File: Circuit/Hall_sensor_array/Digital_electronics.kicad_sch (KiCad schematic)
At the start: 17 parts, among them J1 Conn_01x04_Female, U277 4040

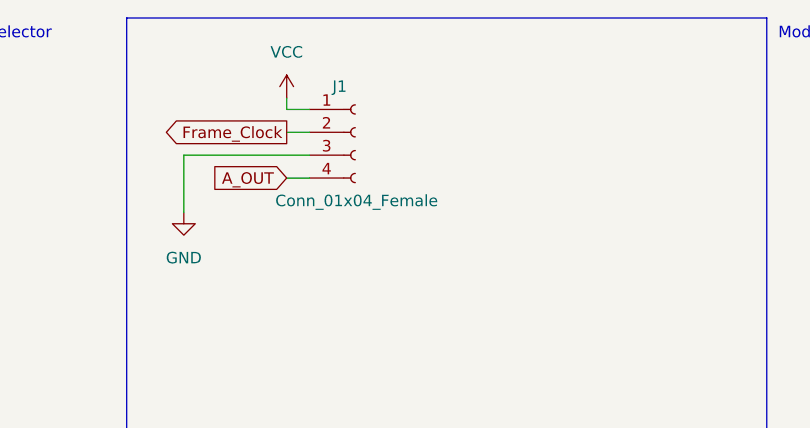
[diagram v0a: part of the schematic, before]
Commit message: Major update! New pcb
i did some work
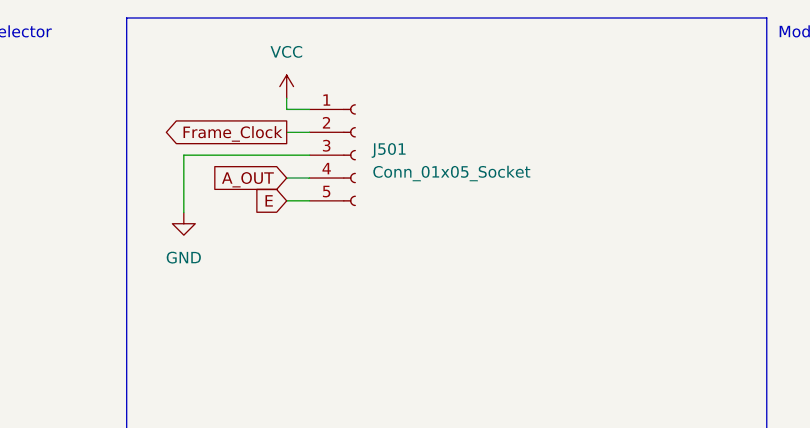
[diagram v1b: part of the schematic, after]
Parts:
- removed J1: Conn_01x04_Female, Connector_PinHeader_2.54mm:PinHeader_1x04_P2.54mm_Horizontal, symbol Connector:Conn_01x04_Female
- added J501: Conn_01x05_Socket, Connector_PinHeader_2.54mm:PinHeader_1x05_P2.54mm_Horizontal, symbol Connector:Conn_01x05_Socket
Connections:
- net A_OUT: now also J501.4 (Pin_4)
- net Frame_Clock: now also J501.2 (Pin_2)
- net GND: now also J501.3 (Pin_3)
- net VCC: now also J501.1 (Pin_1)
- new net E: J501.5 (Pin_5)
